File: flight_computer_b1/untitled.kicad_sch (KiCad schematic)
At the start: 1 part, among them U12 LTC7810

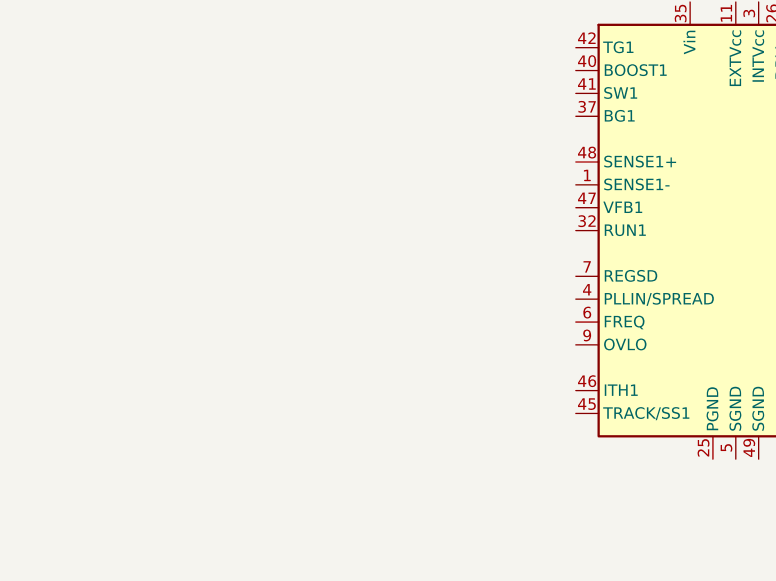
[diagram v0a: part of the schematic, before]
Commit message: WIP
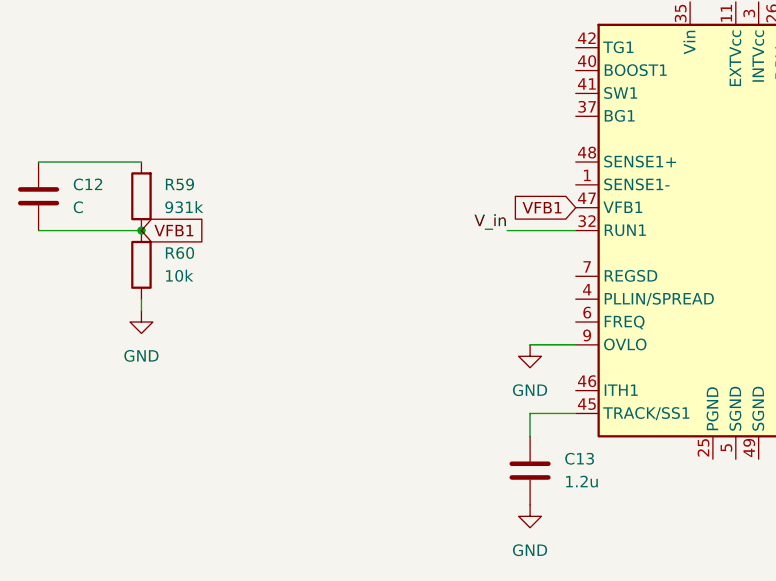
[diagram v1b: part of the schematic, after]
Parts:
- added C12: C, symbol Device:C
- added C13: 1.2u, symbol Device:C
- added R59: 931k, symbol Device:R
- added R60: 10k, symbol Device:R
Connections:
- net V_in: now reaches U12.32 (RUN1)
- net at U12.45 (TRACK/SS1): now also C13.1
- net VFB1: now reaches U12.47 (VFB1)
- net VFB1: now also C12.2, R59.1, R60.2
- net GND: now reaches U12.9 (OVLO)
- net GND: now also C13.2, R60.1
- new net: C12.1, R59.2

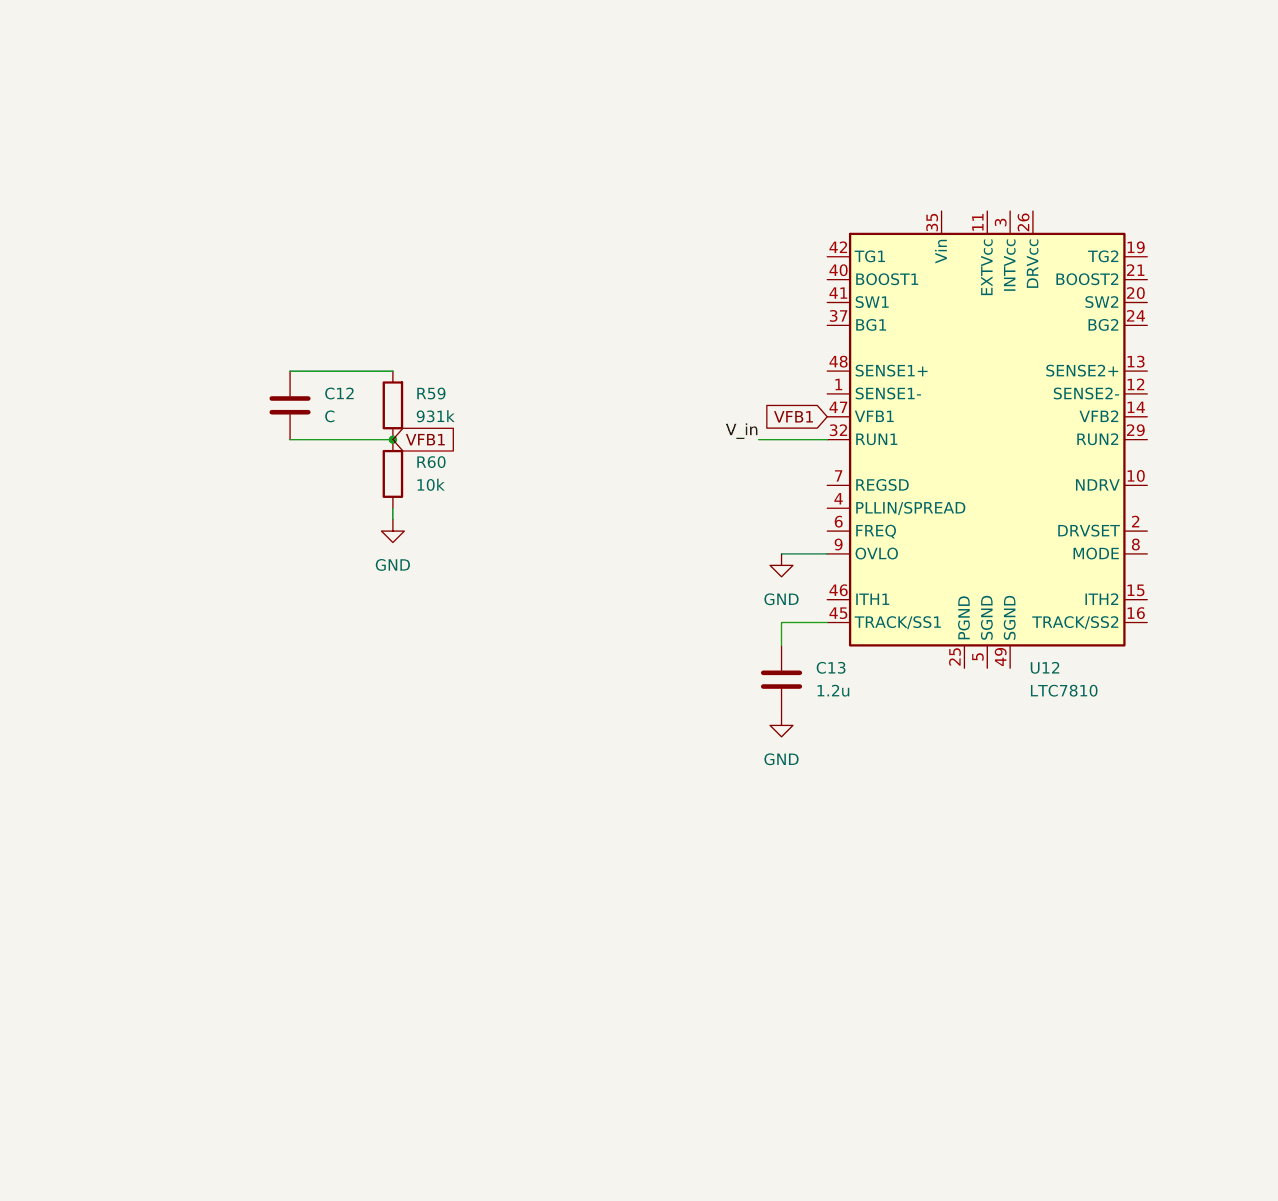
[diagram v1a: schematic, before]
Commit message: vers1
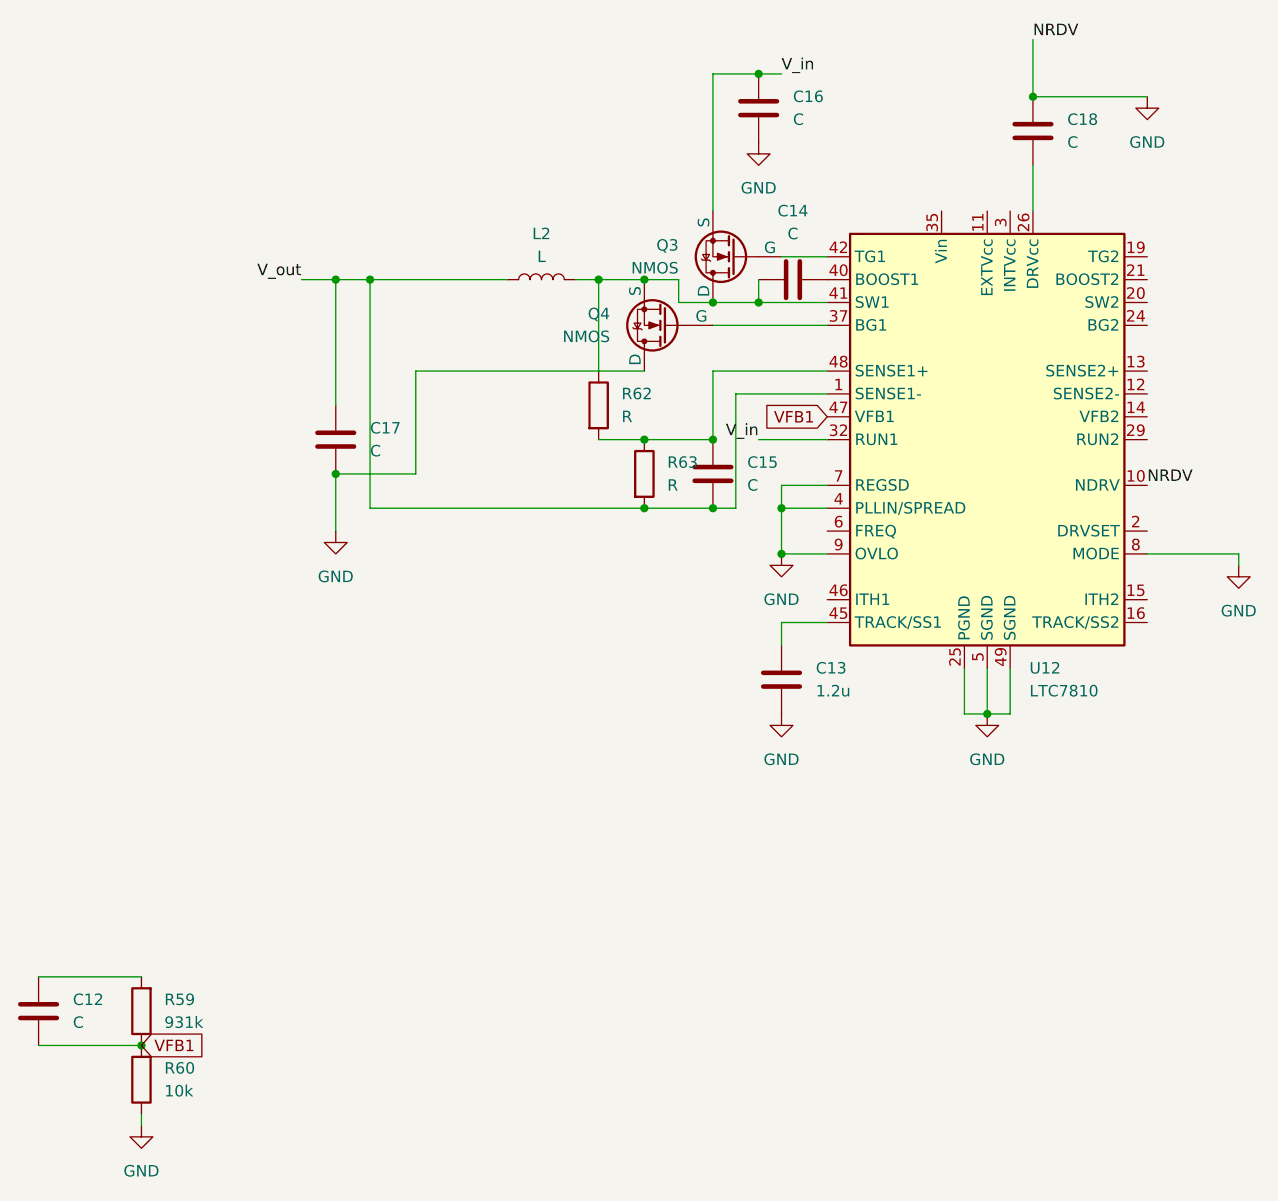
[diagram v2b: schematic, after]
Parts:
- added C14, C15, C16, C17, C18: C, symbol Device:C
- added L2: L, symbol Device:L
- added Q3, Q4: NMOS, symbol Simulation_SPICE:NMOS
- added R62, R63: R, symbol Device:R
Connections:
- net GND: now also U12.10 (NDRV), U12.25 (PGND), U12.4 (PLLIN/SPREAD), U12.49 (SGND), U12.5 (SGND), U12.7 (REGSD), U12.8 (MODE), C16.2, C17.2, C18.1, Q4.1 (D)
- net V_in: now also C16.1, Q3.3 (S)
- net V_out: now reaches U12.1 (SENSE1-)
- net V_out: now also C15.2, C17.1, L2.1, R63.2
- net at U12.26 (DRVcc): now also C18.2
- net at U12.37 (BG1): now also Q4.2 (G)
- net at U12.40 (BOOST1): now also C14.2
- net at U12.41 (SW1): now also C14.1, L2.2, Q3.1 (D), Q4.3 (S), R62.1
- net at U12.42 (TG1): now also Q3.2 (G)
- net at U12.48 (SENSE1+): now also C15.1, R62.2, R63.1
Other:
- moved on the sheet: C12, R59, R60
